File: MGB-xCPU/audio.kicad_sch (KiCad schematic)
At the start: 39 parts, among them P5 Headphones, U3 IR3R53N

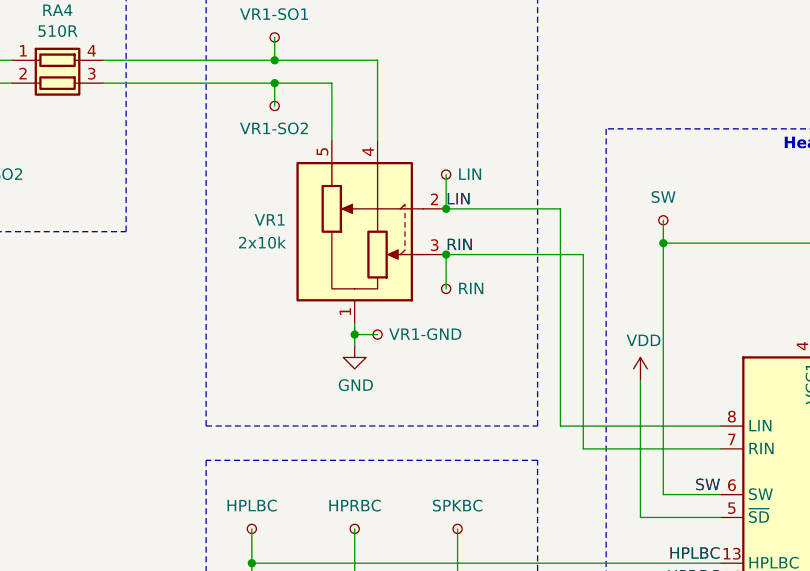
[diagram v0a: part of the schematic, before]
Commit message: Tidy up potentiometer symbols, add contrast pot symbols
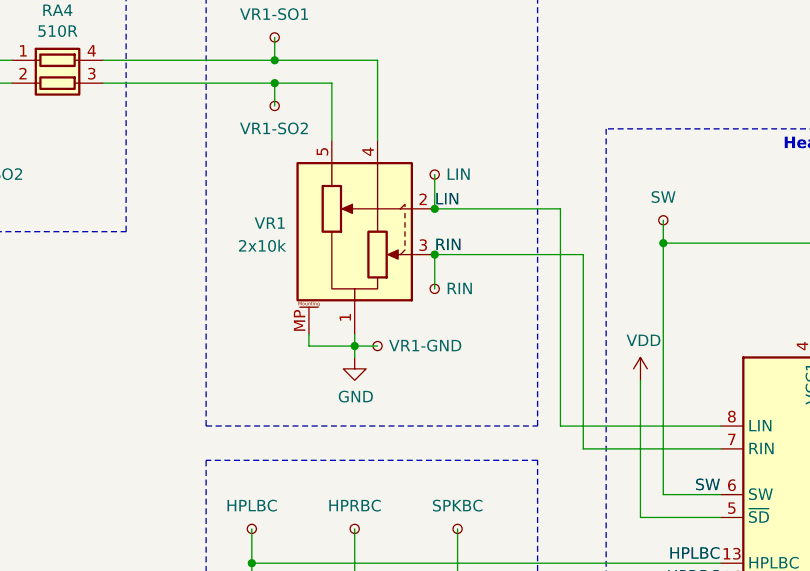
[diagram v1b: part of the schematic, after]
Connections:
- net GND: now also VR1.MP (MountPin)
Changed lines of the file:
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@@
   (junction (at 39.37 71.12) (diameter 0) (color 0 0 0 0)
   )
-  (junction (at 90.17 85.09) (diameter 0) (color 0 0 0 0)
+  (junction (at 88.9 80.01) (diameter 0) (color 0 0 0 0)
   )
   (junction (at 68.58 119.38) (diameter 0) (color 0 0 0 0)
@@
   (junction (at 187.96 106.68) (diameter 0) (color 0 0 0 0)
   )
-  (junction (at 90.17 80.01) (diameter 0) (color 0 0 0 0)
-  )
   (junction (at 80.01 133.35) (diameter 0) (color 0 0 0 0)
   )
@@
   (junction (at 71.12 66.04) (diameter 0) (color 0 0 0 0)
   )
-  (junction (at 80.01 93.98) (diameter 0) (color 0 0 0 0)
+  (junction (at 80.01 95.25) (diameter 0) (color 0 0 0 0)
   )
   (junction (at 243.84 57.15) (diameter 0) (color 0 0 0 0)
@@
   (junction (at 210.82 57.15) (diameter 0) (color 0 0 0 0)
   )
+  (junction (at 88.9 85.09) (diameter 0) (color 0 0 0 0)
+  )
   (junction (at 176.53 125.73) (diameter 0) (color 0 0 0 0)
   )
   (junction (at 71.12 63.5) (diameter 0) (color 0 0 0 0)
   )
-  (wire (pts (xy 80.01 93.98) (xy 82.55 93.98))
+  (wire (pts (xy 80.01 95.25) (xy 82.55 95.25))
     (stroke (width 0) (type default))
   )
@@
     (stroke (width 0) (type default))
   )
+  (wire (pts (xy 74.93 95.25) (xy 80.01 95.25))
+    (stroke (width 0) (type default))
+  )
   (wire (pts (xy 39.37 55.88) (xy 39.37 58.42))
     (stroke (width 0) (type default))
@@
     (stroke (width 0) (type default))
   )
-  (wire (pts (xy 90.17 85.09) (xy 105.41 85.09))
+  (wire (pts (xy 88.9 85.09) (xy 105.41 85.09))
     (stroke (width 0) (type default))
   )
@@
     (stroke (width 0) (type default))
   )
-  (wire (pts (xy 80.01 92.71) (xy 80.01 93.98))
-    (stroke (width 0) (type default))
-  )
   (polyline (pts (xy 160.02 71.12) (xy 107.95 71.12))
     (stroke (width 0) (type dash))
@@
     (stroke (width 0) (type default))
   )
-  (wire (pts (xy 80.01 93.98) (xy 80.01 95.25))
+  (wire (pts (xy 80.01 95.25) (xy 80.01 96.52))
     (stroke (width 0) (type default))
   )
@@
     (stroke (width 0) (type default))
   )
+  (wire (pts (xy 80.01 95.25) (xy 80.01 93.98))
+    (stroke (width 0) (type default))
+  )
   (wire (pts (xy 255.27 99.06) (xy 252.73 99.06))
     (stroke (width 0) (type default))
@@
     (stroke (width 0) (type default))
   )
-  (wire (pts (xy 90.17 80.01) (xy 102.87 80.01))
+  (wire (pts (xy 88.9 80.01) (xy 102.87 80.01))
     (stroke (width 0) (type default))
   )
@@
     (stroke (width 0) (type default))
   )
+  (wire (pts (xy 74.93 93.98) (xy 74.93 95.25))
+    (stroke (width 0) (type default))
+  )
   (wire (pts (xy 187.96 101.6) (xy 187.96 106.68))
     (stroke (width 0) (type default))
@@
     (stroke (width 0) (type default))
   )
-  (wire (pts (xy 90.17 76.2) (xy 90.17 80.01))
+  (wire (pts (xy 88.9 76.2) (xy 88.9 80.01))
     (stroke (width 0) (type default))
   )
@@
     (stroke (width 0) (type default))
   )
-  (wire (pts (xy 90.17 85.09) (xy 90.17 88.9))
+  (wire (pts (xy 88.9 85.09) (xy 88.9 88.9))
     (stroke (width 0) (type default))
   )
@@
     (effects (font (size 1.27 1.27)) (justify left bottom))
   )
-  (label "RIN" (at 90.17 85.09 0) (fields_autoplaced)
+  (label "RIN" (at 88.9 85.09 0) (fields_autoplaced)
     (effects (font (size 1.27 1.27)) (justify left bottom))
   )
-  (label "LIN" (at 90.17 80.01 0) (fields_autoplaced)
+  (label "LIN" (at 88.9 80.01 0) (fields_autoplaced)
     (effects (font (size 1.27 1.27)) (justify left bottom))
   )
@@
     )
   )
-  (symbol (lib_id "Connector:TestPoint_Small") (at 82.55 93.98 0) (unit 1)
-    (in_bom yes) (on_board yes) (dnp no)
-    (property "Reference" "TP48" (at 83.7692 92.8116 0)
+  (symbol (lib_id "Connector:TestPoint_Small") (at 82.55 95.25 0) (unit 1)
+    (in_bom yes) (on_board yes) (dnp no)
+    (property "Reference" "TP48" (at 83.7692 94.0816 0)
       (effects (font (size 1.27 1.27)) (justify left) hide)
     )
-    (property "Value" "VR1-GND" (at 83.82 93.9799 0)
-      (effects (font (size 1.27 1.27)) (justify left))
-    )
-    (property "Footprint" "" (at 87.63 93.98 0)
-      (effects (font (size 1.27 1.27)) hide)
-    )
-    (property "Datasheet" "~" (at 87.63 93.98 0)
+    (property "Value" "VR1-GND" (at 83.82 95.2499 0)
+      (effects (font (size 1.27 1.27)) (justify left))
+    )
+    (property "Footprint" "" (at 87.63 95.25 0)
+      (effects (font (size 1.27 1.27)) hide)
+    )
+    (property "Datasheet" "~" (at 87.63 95.25 0)
       (effects (font (size 1.27 1.27)) hide)
     )
@@
     )
   )
-  (symbol (lib_id "Connector:TestPoint_Small") (at 90.17 76.2 180) (unit 1)
-    (in_bom yes) (on_board yes) (dnp no) (fields_autoplaced)
-    (property "Reference" "TP47" (at 85.471 76.2 90)
-      (effects (font (size 1.27 1.27)) hide)
-    )
-    (property "Value" "LIN" (at 91.44 76.1999 0)
+  (symbol (lib_id "Connector:TestPoint_Small") (at 88.9 76.2 180) (unit 1)
+    (in_bom yes) (on_board yes) (dnp no) (fields_autoplaced)
+    (property "Reference" "TP47" (at 84.201 76.2 90)
+      (effects (font (size 1.27 1.27)) hide)
+    )
+    (property "Value" "LIN" (at 90.17 76.1999 0)
       (effects (font (size 1.27 1.27)) (justify right))
     )
-    (property "Footprint" "" (at 85.09 76.2 0)
-      (effects (font (size 1.27 1.27)) hide)
-    )
-    (property "Datasheet" "~" (at 85.09 76.2 0)
+    (property "Footprint" "" (at 83.82 76.2 0)
+      (effects (font (size 1.27 1.27)) hide)
+    )
+    (property "Datasheet" "~" (at 83.82 76.2 0)
       (effects (font (size 1.27 1.27)) hide)
     )
@@
     )
   )
-  (symbol (lib_id "Connector:TestPoint_Small") (at 90.17 88.9 180) (unit 1)
-    (in_bom yes) (on_board yes) (dnp no) (fields_autoplaced)
-    (property "Reference" "TP51" (at 85.471 88.9 90)
-      (effects (font (size 1.27 1.27)) hide)
-    )
-    (property "Value" "RIN" (at 91.44 88.8999 0)
+  (symbol (lib_id "Connector:TestPoint_Small") (at 88.9 88.9 180) (unit 1)
+    (in_bom yes) (on_board yes) (dnp no)
+    (property "Reference" "TP51" (at 84.201 88.9 90)
+      (effects (font (size 1.27 1.27)) hide)
+    )
+    (property "Value" "RIN" (at 90.17 88.8999 0)
       (effects (font (size 1.27 1.27)) (justify right))
     )
-    (property "Footprint" "" (at 85.09 88.9 0)
-      (effects (font (size 1.27 1.27)) hide)
-    )
-    (property "Datasheet" "~" (at 85.09 88.9 0)
+    (property "Footprint" "" (at 83.82 88.9 0)
+      (effects (font (size 1.27 1.27)) hide)
+    )
+    (property "Datasheet" "~" (at 83.82 88.9 0)
       (effects (font (size 1.27 1.27)) hide)
     )
@@
     )
   )
-  (symbol (lib_id "Gekkio_Device_Specialized:R_Potentiometer_GameBoy_Volume_MGB") (at 80.01 82.55 270) (mirror x) (unit 1)
-    (in_bom yes) (on_board yes) (dnp no) (fields_autoplaced)
-    (property "Reference" "VR1" (at 72.39 81.2799 90)
-      (effects (font (size 1.27 1.27)) (justify right))
-    )
-    (property "Value" "2x10k" (at 72.39 83.8199 90)
-      (effects (font (size 1.27 1.27)) (justify right))
-    )
-    (property "Footprint" "" (at 78.105 78.74 0)
-      (effects (font (size 1.27 1.27)) hide)
-    )
-    (property "Datasheet" "~" (at 78.105 78.74 0)
+  (symbol (lib_id "Gekkio_Device_Specialized:R_Potentiometer_GameBoy_Volume_MGB") (at 80.01 82.55 0) (mirror y) (unit 1)
+    (in_bom yes) (on_board yes) (dnp no) (fields_autoplaced)
+    (property "Reference" "VR1" (at 72.39 81.6356 0)
+      (effects (font (size 1.27 1.27)) (justify left))
+    )
+    (property "Value" "2x10k" (at 72.39 84.1756 0)
+      (effects (font (size 1.27 1.27)) (justify left))
+    )
+    (property "Footprint" "" (at 76.2 84.455 0)
+      (effects (font (size 1.27 1.27)) hide)
+    )
+    (property "Datasheet" "~" (at 76.2 84.455 0)
       (effects (font (size 1.27 1.27)) hide)
     )
@@
     (pin "4")
     (pin "5")
+    (pin "MP")
     (instances
       (project "MGB-xCPU"
@@
     )
   )
-  (symbol (lib_id "power:GND") (at 80.01 95.25 0) (unit 1)
-    (in_bom yes) (on_board yes) (dnp no)
-    (property "Reference" "#PWR0134" (at 80.01 101.6 0)
-      (effects (font (size 1.27 1.27)) hide)
-    )
-    (property "Value" "GND" (at 80.137 99.6442 0)
-      (effects (font (size 1.27 1.27)))
-    )
-    (property "Footprint" "" (at 80.01 95.25 0)
-      (effects (font (size 1.27 1.27)) hide)
-    )
-    (property "Datasheet" "" (at 80.01 95.25 0)
-      (effects (font (size 1.27 1.27)) hide)
-    )
+  (symbol (lib_id "power:GND") (at 80.01 96.52 0) (unit 1)
+    (in_bom yes) (on_board yes) (dnp no)
+    (property "Reference" "#PWR0134" (at 80.01 102.87 0)
+      (effects (font (size 1.27 1.27)) hide)
+    )
+    (property "Value" "GND" (at 80.137 100.9142 0)
+      (effects (font (size 1.27 1.27)))
+    )
+    (property "Footprint" "" (at 80.01 96.52 0)
+      (effects (font (size 1.27 1.27)) hide)
+    )
+    (property "Datasheet" "" (at 80.01 96.52 0)
+      (effects (font (size 1.27 1.27)) hide)
+    )
